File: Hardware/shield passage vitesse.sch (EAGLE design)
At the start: 37 parts, among them Q1 2N7000, Q2 2N7000, Q3 2N7000, Q4 2N7000, Q5 2N7000

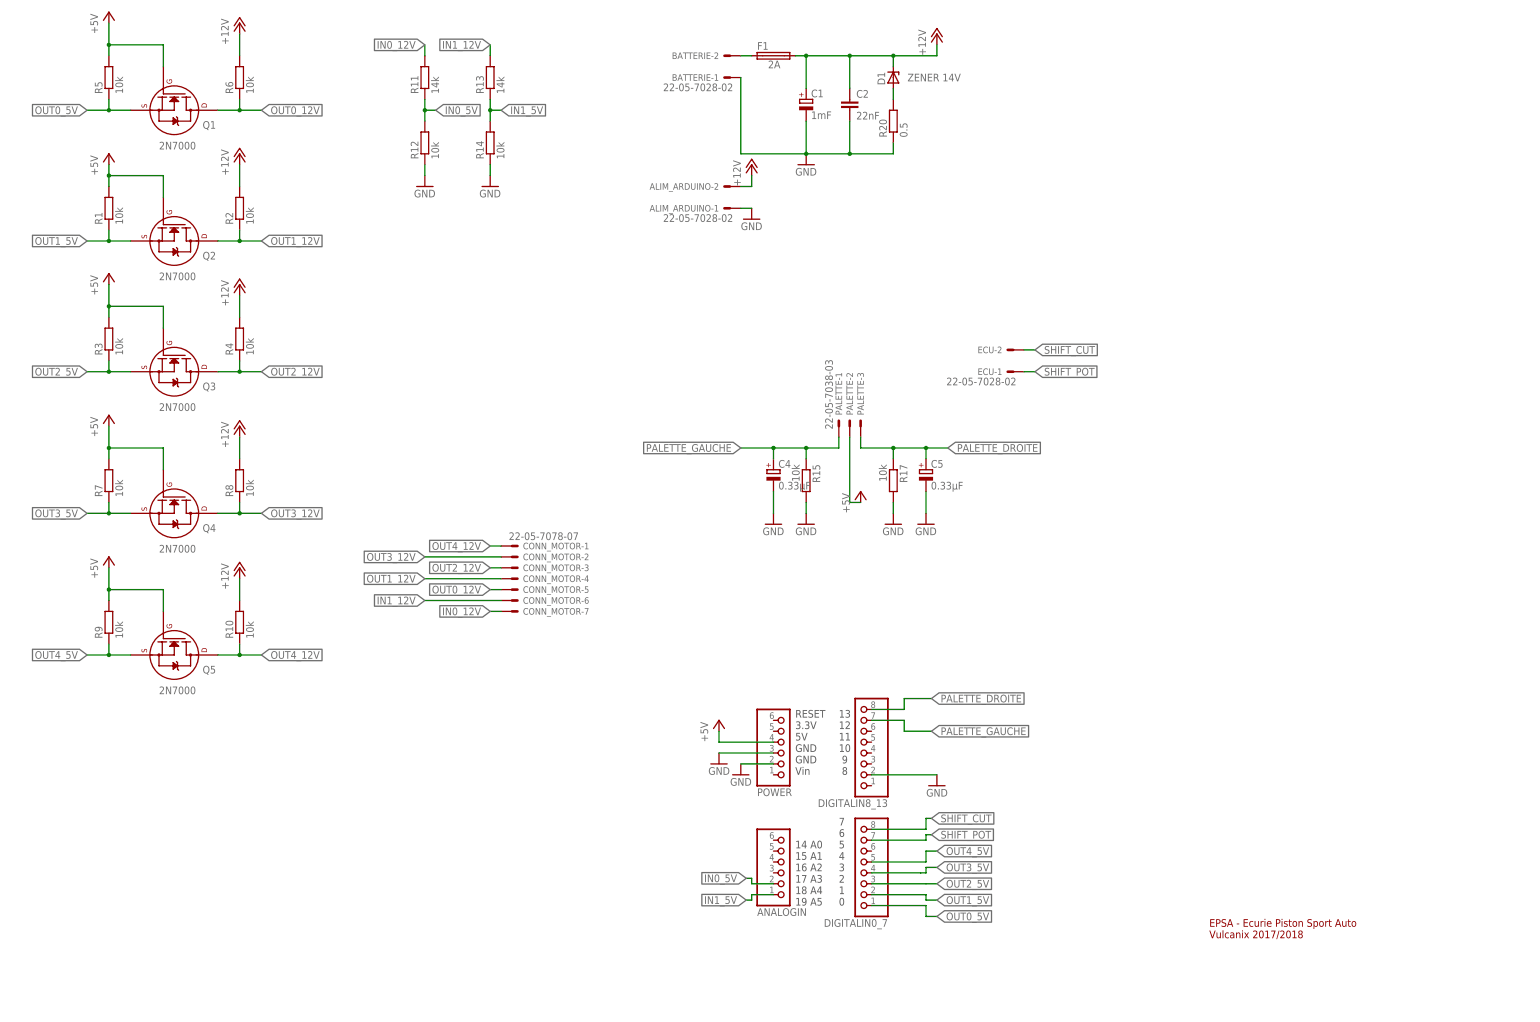
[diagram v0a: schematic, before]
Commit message: Mise en qualité
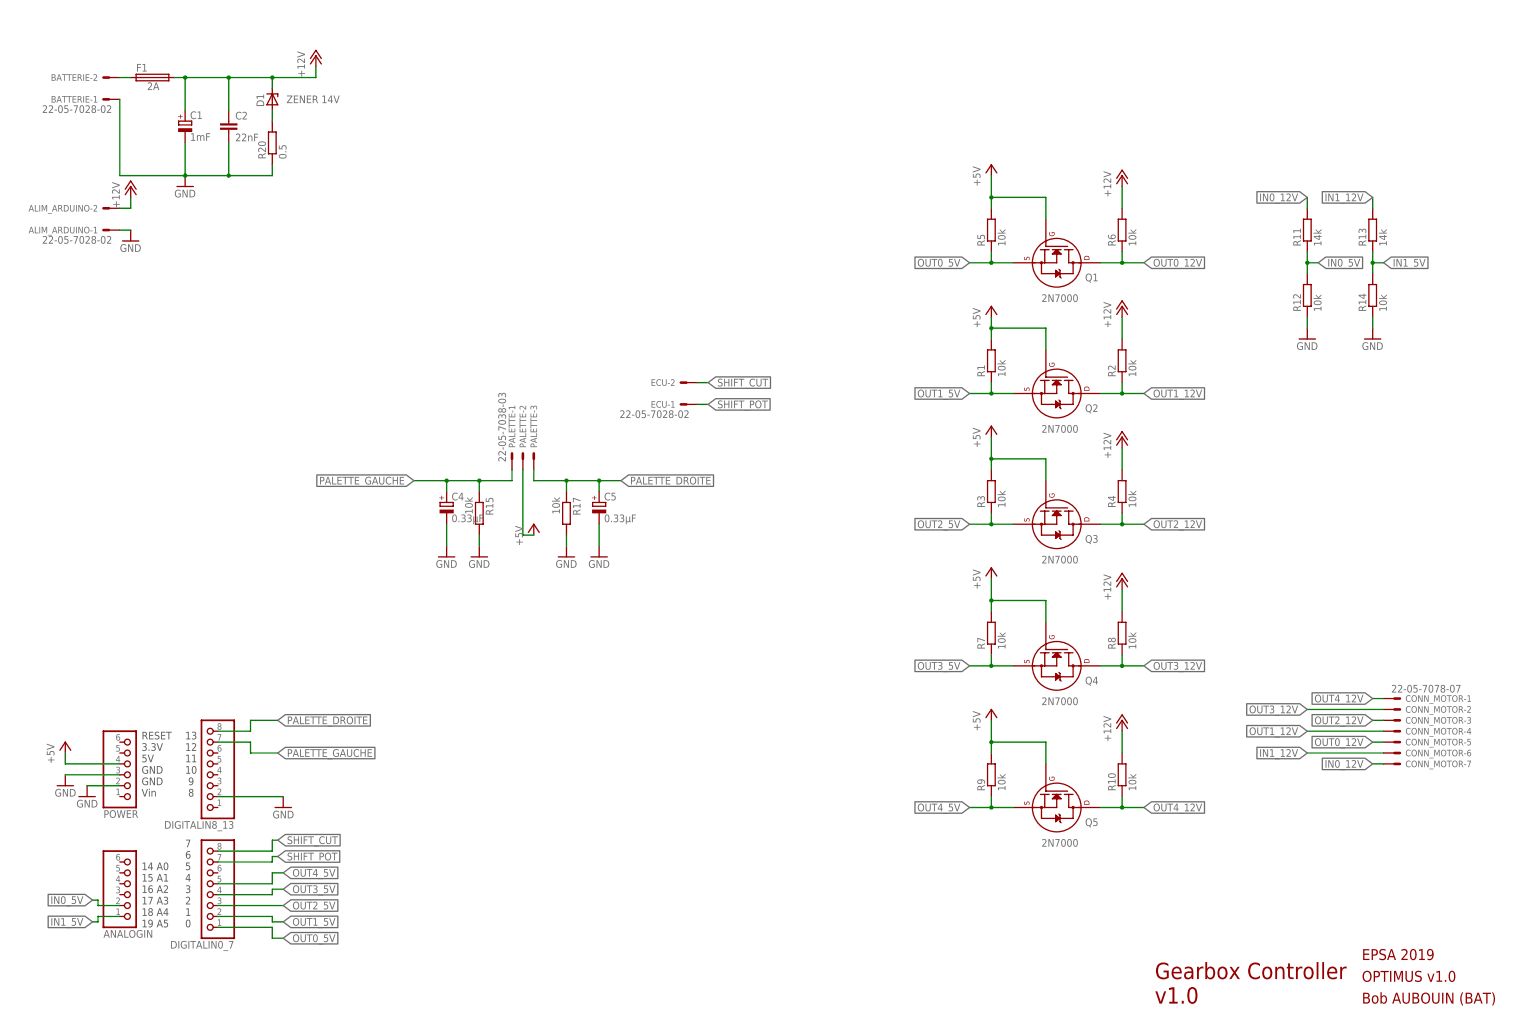
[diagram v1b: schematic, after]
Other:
- note added: "Bob AUBOUIN (BAT)"
- note added: "EPSA 2019"
- note added: "Gearbox Controller v1.0"
- note added: "OPTIMUS v1.0"
- note removed: "EPSA - Ecurie Piston Sport Auto Vulcanix 2017/2018"
- moved on the sheet: ALIM_ARDUINO-1, ALIM_ARDUINO-2, ANALOGIN, BATTERIE-1, BATTERIE-2, C1, C2, C4, C5, CONN_MOTOR-1, CONN_MOTOR-2, CONN_MOTOR-3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
